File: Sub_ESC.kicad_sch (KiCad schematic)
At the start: 2 parts

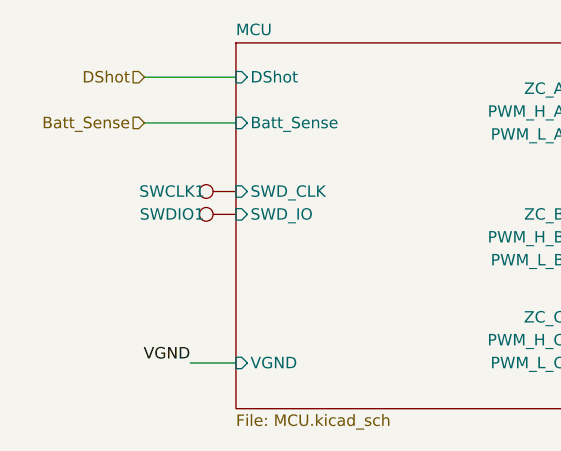
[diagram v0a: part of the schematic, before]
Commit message: more routing and placement
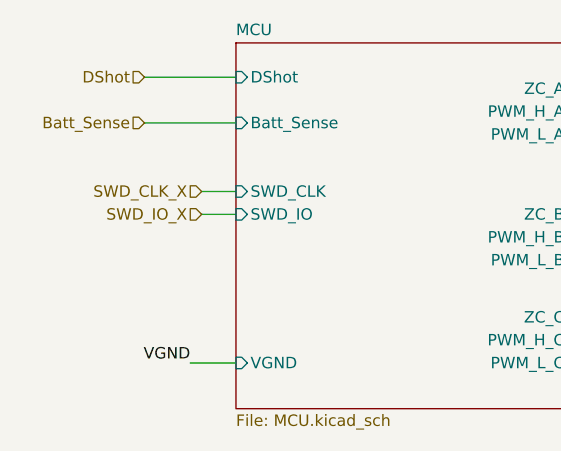
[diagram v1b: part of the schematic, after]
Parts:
- removed SWCLK1, SWDIO1: TestPoint, TestPoint:TestPoint_Pad_1.0x1.0mm, symbol Connector:TestPoint
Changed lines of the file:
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@@
+	(wire
+		(pts
+			(xy 73.66 93.98) (xy 77.47 93.98)
+		)
+		(stroke
+			(width 0)
+			(type default)
+		)
+	)
 	(wire
 		(pts
@@
 		(pts
 			(xy 115.57 105.41) (xy 175.26 105.41)
+		)
+		(stroke
+			(width 0)
+			(type default)
+		)
+	)
+	(wire
+		(pts
+			(xy 73.66 91.44) (xy 77.47 91.44)
 		)
 		(stroke
@@
 		)
 	)
+	(hierarchical_label "SWD_CLK_X"
+		(shape input)
+		(at 73.66 91.44 180)
+		(effects
+			(font
+				(size 1.27 1.27)
+			)
+			(justify right)
+		)
+	)
 	(hierarchical_label "Batt_Sense"
 		(shape input)
@@
 		)
 	)
-	(symbol
-		(lib_id "Connector:TestPoint")
-		(at 77.47 91.44 90)
-		(unit 1)
-		(exclude_from_sim no)
-		(in_bom yes)
-		(on_board yes)
-		(dnp no)
-		(property "Reference" "SWCLK1"
-			(at 70.358 91.44 90)
-			(effects
-				(font
-					(size 1.27 1.27)
-				)
-			)
-		)
-		(property "Value" "TestPoint"
-			(at 67.564 90.424 90)
-			(effects
-				(font
-					(size 1.27 1.27)
-				)
-				(hide yes)
-			)
-		)
-		(property "Footprint" "TestPoint:TestPoint_Pad_1.0x1.0mm"
-			(at 77.47 86.36 0)
-			(effects
-				(font
-					(size 1.27 1.27)
-				)
-				(hide yes)
-			)
-		)
-		(property "Datasheet" "~"
-			(at 77.47 86.36 0)
-			(effects
-				(font
-					(size 1.27 1.27)
-				)
-				(hide yes)
-			)
-		)
-		(property "Description" "test point"
-			(at 77.47 91.44 0)
-			(effects
-				(font
-					(size 1.27 1.27)
-				)
-				(hide yes)
-			)
-		)
-		(pin "1"
-		)
-		(instances
-			(project ""
-				(path "/0e826802-e676-4548-b85d-7973e5fc1500/dd4480c0-fc92-4865-b71a-49548ede0e1d"
-					(reference "SWCLK1")
-					(unit 1)
-				)
-			)
-		)
-	)
-	(symbol
-		(lib_id "Connector:TestPoint")
-		(at 77.47 93.98 90)
-		(unit 1)
-		(exclude_from_sim no)
-		(in_bom yes)
-		(on_board yes)
-		(dnp no)
-		(property "Reference" "SWDIO1"
-			(at 70.358 93.98 90)
-			(effects
-				(font
-					(size 1.27 1.27)
-				)
-			)
-		)
-		(property "Value" "TestPoint"
-			(at 74.168 91.44 90)
-			(effects
-				(font
-					(size 1.27 1.27)
-				)
-				(hide yes)
-			)
-		)
-		(property "Footprint" "TestPoint:TestPoint_Pad_1.0x1.0mm"
-			(at 77.47 88.9 0)
-			(effects
-				(font
-					(size 1.27 1.27)
-				)
-				(hide yes)
-			)
-		)
-		(property "Datasheet" "~"
-			(at 77.47 88.9 0)
-			(effects
-				(font
-					(size 1.27 1.27)
-				)
-				(hide yes)
-			)
-		)
-		(property "Description" "test point"
-			(at 77.47 93.98 0)
-			(effects
-				(font
-					(size 1.27 1.27)
-				)
-				(hide yes)
-			)
-		)
-		(pin "1"
-		)
-		(instances
-			(project ""
-				(path "/0e826802-e676-4548-b85d-7973e5fc1500/dd4480c0-fc92-4865-b71a-49548ede0e1d"
-					(reference "SWDIO1")
-					(unit 1)
-				)
-			)
+	(hierarchical_label "SWD_IO_X"
+		(shape input)
+		(at 73.66 93.98 180)
+		(effects
+			(font
+				(size 1.27 1.27)
+			)
+			(justify right)
 		)
 	)
@@
 					(page "3")
 				)
+				(path "/0e826802-e676-4548-b85d-7973e5fc1500/67868d63-a0ad-4135-884b-a4305faec098"
+					(page "10")
+				)
+				(path "/0e826802-e676-4548-b85d-7973e5fc1500/f0f91033-e6f6-4ba6-a242-b2d52399ba4f"
+					(page "16")
+				)
+				(path "/0e826802-e676-4548-b85d-7973e5fc1500/e90d83da-778a-41e9-b4cb-1e16efdba290"
+					(page "22")
+				)
 			)
 		)
@@
 					(page "7")
 				)
-			)
+				(path "/0e826802-e676-4548-b85d-7973e5fc1500/67868d63-a0ad-4135-884b-a4305faec098"
+					(page "14")
+				)
+				(path "/0e826802-e676-4548-b85d-7973e5fc1500/f0f91033-e6f6-4ba6-a242-b2d52399ba4f"
+					(page "20")
+				)
+				(path "/0e826802-e676-4548-b85d-7973e5fc1500/e90d83da-778a-41e9-b4cb-1e16efdba290"
+					(page "26")
+				)
+			)
